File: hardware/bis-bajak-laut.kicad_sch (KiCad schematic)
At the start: 253 parts, among them J1 TFT, J2 USB_C_Receptacle_USB2.0_14P, J3 ProgHeader, J4 BIS BAJAK LAUT IO, J5 BIS BAJAK LAUT IO, Q1 SI2301, Q10 SI2301, Q11 MMBT3906, Q12 BCM857, Q13 MMBT3906, Q14 SI2301, Q2 SI2301, Q3 SI2301, Q4 SI2301, Q5 SI2301, Q6 SI2301, Q7 SI2301, Q8 MMBT7002K, Q9 SI2301, SW1 W25Sel, SW2 BUTTON, U1 MT29F1G01ABAFDWB, U10 LMV331, U11 AP2127K-ADJ, U12 LMV321, U13 LMV321, U14 W25Q128JVS, U15 AMS1117-3.3, U16 SN74LVC1T45DRL, U17 SN74LVC1T45DRL, U18 SN74LVC1T45DRL, U19 SN74LVC1T45DRL, U2 74HC595, U20 SN74LVC1T45DRL, U21 SN74LVC1T45DRL, U22 SN74LVC1T45DRL, U23 SN74LVC1T45DRL, U3 LMV324, U4 CD74HC4067M, U5 74HC245, U6 74HC595, U7 LMV324, U8 LMV324, U9 RP2040, Y1 12Mhz

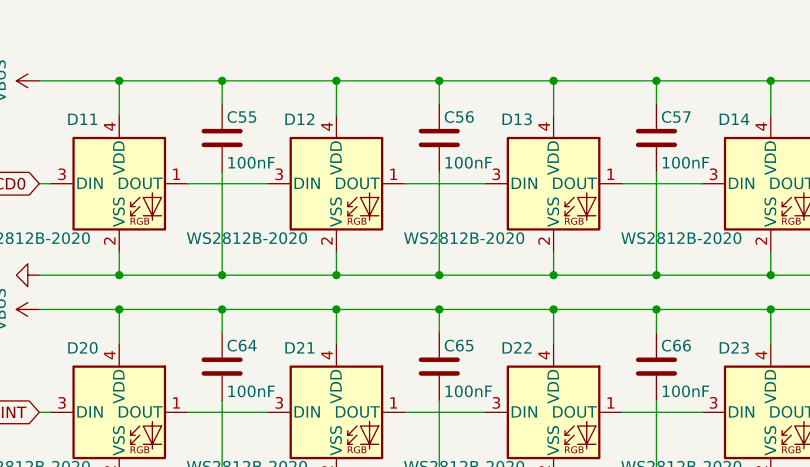
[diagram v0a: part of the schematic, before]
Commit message: feat: component arrangement progress 1
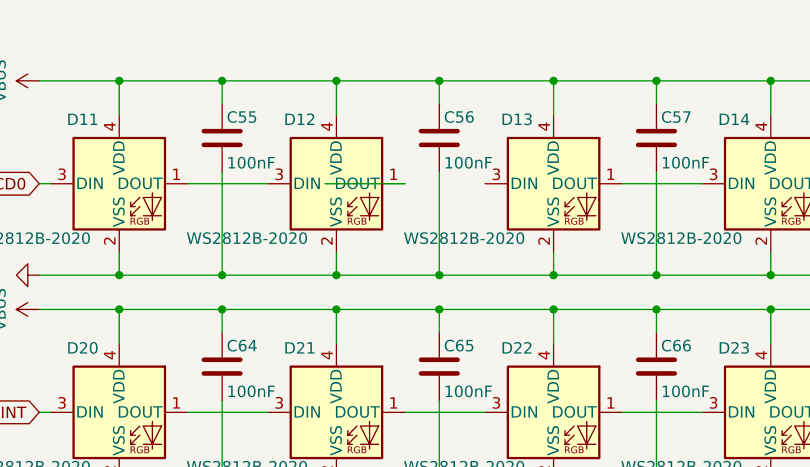
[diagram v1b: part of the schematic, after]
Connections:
- net at D13.3 (DIN): no longer D12.1 (DOUT)
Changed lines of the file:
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@@
 	(wire
 		(pts
-			(xy 69.85 30.48) (xy 78.74 30.48)
+			(xy 69.85 30.48) (xy 60.96 30.48)
 		)
 		(stroke
